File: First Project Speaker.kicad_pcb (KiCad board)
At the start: 2 copper layers, 63.5 x 66.7 mm, 55 parts, among them J1 USB_C_Receptacle_USB2.0_16P, J2 Screw_Terminal_01x02, J3 Screw_Terminal_01x02, SW1 SW_Push, SW2 SW_Push, SW3 SW_Push, U1 LD1117S33TR_SOT223, U2 PCM2704CDBR, U3 TDA7297, U4 CH221K, Y1 12M

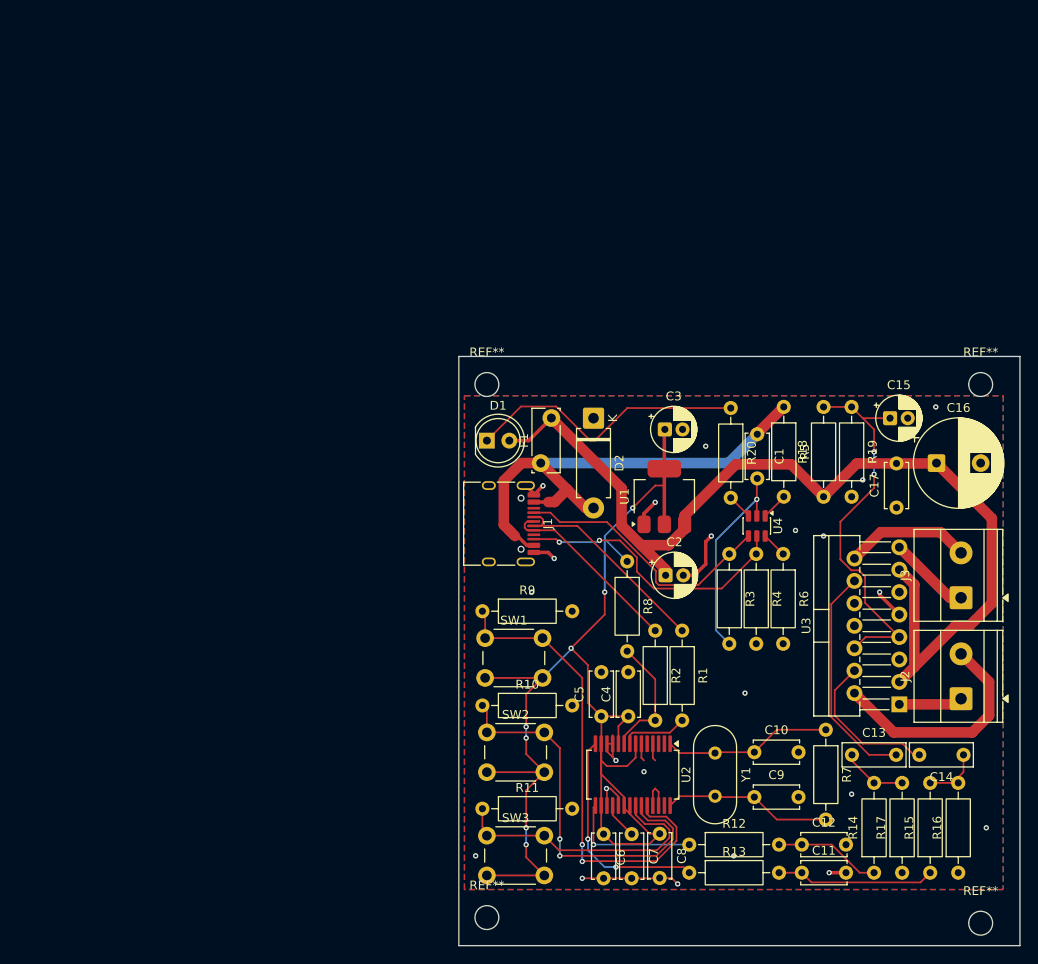
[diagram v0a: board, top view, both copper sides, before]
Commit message: V2: SMD/0805 passives, side buttons, envelope-detector visualizer planning
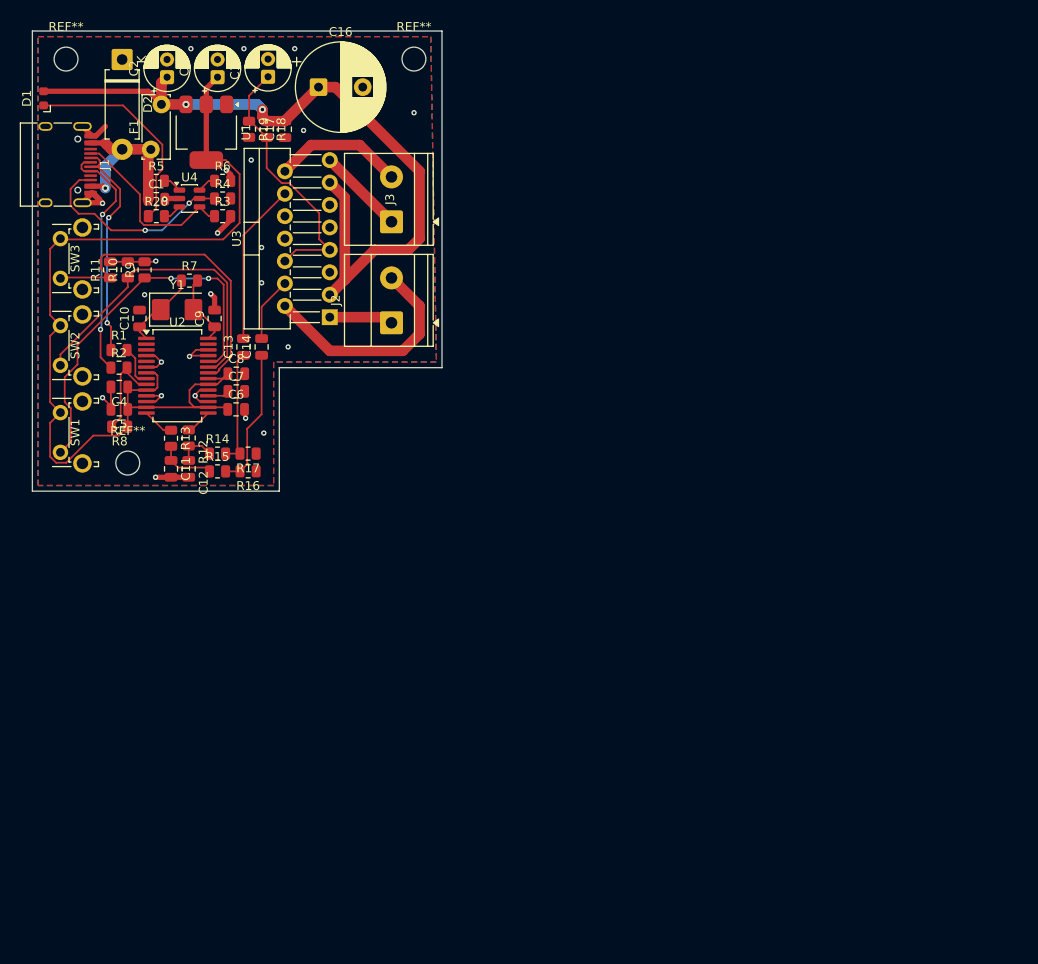
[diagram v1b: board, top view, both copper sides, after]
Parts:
- removed the REF** at (174.6, 132.7)
- C1, C10, C11, C12, C17, C4, C5, C6, C7, C8, C9: footprint Capacitor_THT:C_Disc_D5.0mm_W2.5mm_P5.00mm -> Capacitor_SMD:C_0805_2012Metric
- C13, C14: footprint Capacitor_THT:C_Rect_L7.0mm_W2.5mm_P5.00mm -> Capacitor_SMD:C_0805_2012Metric
- D1: footprint LED_THT:LED_D5.0mm -> LED_SMD:LED_Kingbright_APA1606_1.6x0.6mm_Horizontal
- R1, R10, R11, R12, R13, R14, R15, R16, R17, R18, R19, R2, R20, R3, R4, R5, R6, R7, R8, R9: footprint Resistor_THT:R_Axial_DIN0207_L6.3mm_D2.5mm_P10.16mm_Horizontal -> Resistor_SMD:R_0805_2012Metric
- SW1, SW2, SW3: footprint Button_Switch_THT:SW_PUSH_6mm -> Button_Switch_THT:SW_Tactile_SPST_Angled_PTS645Vx58-2LFS
- Y1: footprint Crystal:Crystal_HC49-U_Vertical -> Crystal:Crystal_SMD_5032-2Pin_5.0x3.2mm
- moved R15 92.6 mm to (88.3, 81.6), turned to 0 degrees
- moved R16 92.3 mm to (91.7, 81.6), turned to 180 degrees
- moved C14 91.9 mm to (93.2, 67.5), turned to 90 degrees
- moved R14 88.1 mm to (88.3, 79.6), turned to 0 degrees
- moved R7 88.1 mm to (85.1, 60.0), turned to 0 degrees
- moved R17 87.9 mm to (91.7, 79.6), turned to 180 degrees
- moved C10 85.1 mm to (79.4, 64.3), turned to 90 degrees
- moved C11 84.8 mm to (83.0, 81.3), turned to -90 degrees
- moved C13 82.9 mm to (91.2, 67.5), turned to 90 degrees
- moved C16 81.9 mm to (99.7, 38.1)
- moved C9 81.6 mm to (87.9, 64.3), turned to 90 degrees
- moved C17 81.4 mm to (95.9, 42.9)
- moved C12 81.4 mm to (85.0, 81.3), turned to -90 degrees
- moved C15 80.3 mm to (94.0, 36.9), turned to 90 degrees
- moved C2 79.8 mm to (82.5, 37.0), turned to 90 degrees
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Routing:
- net /VBUS_RAW: track 57.5 -> 19.8 mm, vias 0 -> 1
- net /+3.3V: track 146.8 -> 113.3 mm, vias 8 -> 0
- net /+12V: track 114.5 -> 85.4 mm, vias 0 -> 2
- net GND: track 73.6 -> 48.2 mm, vias 22 -> 24
- net Net-(U2-VOUTL): track 24.9 -> 3.59 mm, vias 2 -> 0
- net Net-(U3A-MUTE): track 43.8 -> 30.5 mm, vias 2 -> 0
- net Net-(U2-VOUTR): track 15.3 -> 3.00 mm, vias 1 -> 0
- net /Audio_L: track 18.0 -> 6.46 mm
- net Net-(U2-HID2/MD): track 54.9 -> 43.5 mm
- net Net-(J1-CC1): track 31.3 -> 20.4 mm
- net Net-(U2-XTI): track 19.2 -> 8.28 mm
- net Net-(U3A-+): track 17.7 -> 7.32 mm
- net Net-(U2-XTO): track 19.2 -> 9.09 mm
- net Net-(J1-CC2): track 32.9 -> 23.5 mm
- net Net-(C14-Pad1): track 6.60 -> 15.8 mm
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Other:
- board size 63.5 x 66.7 mm -> 46.4 x 52.1 mm
